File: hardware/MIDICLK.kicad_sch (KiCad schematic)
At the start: 32 parts, among them J1 Conn_02x08_Odd_Even, J2 AudioJack3, J3 AudioJack2, J4 AudioJack2, Q1 2N3904, Q2 2N3904, SW1 RotaryEncoder_Switch, U1 ATtiny85-20P, U2 6N138

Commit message: Assign footprints to components
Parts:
- C1, C2, C3: footprint (none) -> Capacitor_THT:C_Disc_D7.5mm_W5.0mm_P7.50mm
- D2, D3: footprint (none) -> LED_THT:LED_D3.0mm
- J1: footprint (none) -> Connector_IDC:IDC-Header_2x08_P2.54mm_Vertical
- J2: footprint (none) -> AudioJacks:Jack_3.5mm_QingPu_WQP-PJ301CM_Vertical
- J3, J4: footprint (none) -> AudioJacks:Jack_3.5mm_QingPu_WQP-PJ301M-12_Vertical
- R1, R10, R11, R12, R13, R14, R15, R16, R17, R2, R3, R4, R5, R6, R7, R8, R9: footprint (none) -> Resistor_THT:R_Axial_DIN0207_L6.3mm_D2.5mm_P10.16mm_Horizontal
- SW1: footprint (none) -> Rotary_Encoder:RotaryEncoder_Alps_EC11E-Switch_Vertical_H20mm
- U1: footprint Package_DIP:DIP-8_W7.62mm -> Package_DIP:DIP-8_W7.62mm_Socket
- U2: footprint (none) -> Package_DIP:DIP-8_W7.62mm_Socket
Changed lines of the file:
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@@
 			)
 		)
-		(property "Footprint" ""
+		(property "Footprint" "Resistor_THT:R_Axial_DIN0207_L6.3mm_D2.5mm_P10.16mm_Horizontal"
 			(at 210.82 112.268 90)
 			(effects
@@
 			)
 		)
-		(property "Footprint" ""
+		(property "Footprint" "Resistor_THT:R_Axial_DIN0207_L6.3mm_D2.5mm_P10.16mm_Horizontal"
 			(at 210.82 50.038 90)
 			(effects
@@
 			)
 		)
-		(property "Footprint" ""
+		(property "Footprint" "Resistor_THT:R_Axial_DIN0207_L6.3mm_D2.5mm_P10.16mm_Horizontal"
 			(at 244.602 120.65 90)
 			(effects
@@
 			)
 		)
-		(property "Footprint" "Package_DIP:DIP-8_W7.62mm"
+		(property "Footprint" "Package_DIP:DIP-8_W7.62mm_Socket"
 			(at 157.48 82.55 0)
 			(effects
@@
 			)
 		)
-		(property "Footprint" ""
+		(property "Footprint" "Resistor_THT:R_Axial_DIN0207_L6.3mm_D2.5mm_P10.16mm_Horizontal"
 			(at 43.18 91.948 90)
 			(effects
@@
 			)
 		)
-		(property "Footprint" ""
+		(property "Footprint" "Rotary_Encoder:RotaryEncoder_Alps_EC11E-Switch_Vertical_H20mm"
 			(at 82.55 88.646 0)
 			(effects
@@
 			)
 		)
-		(property "Footprint" ""
+		(property "Footprint" "LED_THT:LED_D3.0mm"
 			(at 246.38 48.26 0)
 			(effects
@@
 			)
 		)
-		(property "Footprint" ""
+		(property "Footprint" "Connector_IDC:IDC-Header_2x08_P2.54mm_Vertical"
 			(at 90.17 157.48 0)
 			(effects
@@
 			)
 		)
-		(property "Footprint" ""
+		(property "Footprint" "LED_THT:LED_D3.0mm"
 			(at 246.38 110.49 0)
 			(effects
@@
 			)
 		)
-		(property "Footprint" ""
+		(property "Footprint" "Resistor_THT:R_Axial_DIN0207_L6.3mm_D2.5mm_P10.16mm_Horizontal"
 			(at 89.662 38.1 90)
 			(effects
@@
 			)
 		)
-		(property "Footprint" ""
+		(property "Footprint" "AudioJacks:Jack_3.5mm_QingPu_WQP-PJ301CM_Vertical"
 			(at 34.29 38.1 0)
 			(effects
@@
 			)
 		)
-		(property "Footprint" ""
+		(property "Footprint" "Resistor_THT:R_Axial_DIN0207_L6.3mm_D2.5mm_P10.16mm_Horizontal"
 			(at 100.838 102.87 90)
 			(effects
@@
 			)
 		)
-		(property "Footprint" ""
+		(property "Footprint" "Resistor_THT:R_Axial_DIN0207_L6.3mm_D2.5mm_P10.16mm_Horizontal"
 			(at 48.26 36.322 90)
 			(effects
@@
 			)
 		)
-		(property "Footprint" ""
+		(property "Footprint" "Resistor_THT:R_Axial_DIN0207_L6.3mm_D2.5mm_P10.16mm_Horizontal"
 			(at 67.31 93.472 90)
 			(effects
@@
 			)
 		)
-		(property "Footprint" ""
+		(property "Footprint" "AudioJacks:Jack_3.5mm_QingPu_WQP-PJ301M-12_Vertical"
 			(at 260.35 44.45 0)
 			(effects
@@
 			)
 		)
-		(property "Footprint" ""
+		(property "Footprint" "AudioJacks:Jack_3.5mm_QingPu_WQP-PJ301M-12_Vertical"
 			(at 260.35 106.68 0)
 			(effects
@@
 			)
 		)
-		(property "Footprint" ""
+		(property "Footprint" "Resistor_THT:R_Axial_DIN0207_L6.3mm_D2.5mm_P10.16mm_Horizontal"
 			(at 75.438 83.82 90)
 			(effects
@@
 			)
 		)
-		(property "Footprint" ""
+		(property "Footprint" "Package_DIP:DIP-8_W7.62mm_Socket"
 			(at 82.296 49.53 0)
 			(effects
@@
 			)
 		)
-		(property "Footprint" ""
+		(property "Footprint" "Resistor_THT:R_Axial_DIN0207_L6.3mm_D2.5mm_P10.16mm_Horizontal"
 			(at 235.712 102.87 90)
 			(effects
@@
 			)
 		)
-		(property "Footprint" ""
+		(property "Footprint" "Resistor_THT:R_Axial_DIN0207_L6.3mm_D2.5mm_P10.16mm_Horizontal"
 			(at 223.012 29.21 90)
 			(effects
@@
 			)
 		)
-		(property "Footprint" ""
+		(property "Footprint" "Resistor_THT:R_Axial_DIN0207_L6.3mm_D2.5mm_P10.16mm_Horizontal"
 			(at 223.012 91.44 90)
 			(effects
@@
 			)
 		)
-		(property "Footprint" ""
+		(property "Footprint" "Resistor_THT:R_Axial_DIN0207_L6.3mm_D2.5mm_P10.16mm_Horizontal"
 			(at 47.752 83.82 90)
 			(effects
@@
 			)
 		)
-		(property "Footprint" ""
+		(property "Footprint" "Resistor_THT:R_Axial_DIN0207_L6.3mm_D2.5mm_P10.16mm_Horizontal"
 			(at 244.602 58.42 90)
 			(effects
@@
 			)
 		)
-		(property "Footprint" ""
+		(property "Footprint" "Resistor_THT:R_Axial_DIN0207_L6.3mm_D2.5mm_P10.16mm_Horizontal"
 			(at 235.712 58.42 90)
 			(effects
@@
 			)
 		)
-		(property "Footprint" ""
+		(property "Footprint" "Resistor_THT:R_Axial_DIN0207_L6.3mm_D2.5mm_P10.16mm_Horizontal"
 			(at 235.712 40.64 90)
 			(effects
@@
 			)
 		)
-		(property "Footprint" ""
+		(property "Footprint" "Capacitor_THT:C_Disc_D7.5mm_W5.0mm_P7.50mm"
 			(at 35.8648 106.68 0)
 			(effects
@@
 			)
 		)
-		(property "Footprint" ""
+		(property "Footprint" "Capacitor_THT:C_Disc_D7.5mm_W5.0mm_P7.50mm"
 			(at 139.7 96.8248 0)
 			(effects
@@
 			)
 		)
-		(property "Footprint" ""
+		(property "Footprint" "Capacitor_THT:C_Disc_D7.5mm_W5.0mm_P7.50mm"
 			(at 59.9948 106.68 0)
 			(effects
@@
 			)
 		)
-		(property "Footprint" ""
+		(property "Footprint" "Resistor_THT:R_Axial_DIN0207_L6.3mm_D2.5mm_P10.16mm_Horizontal"
 			(at 235.712 120.65 90)
 			(effects

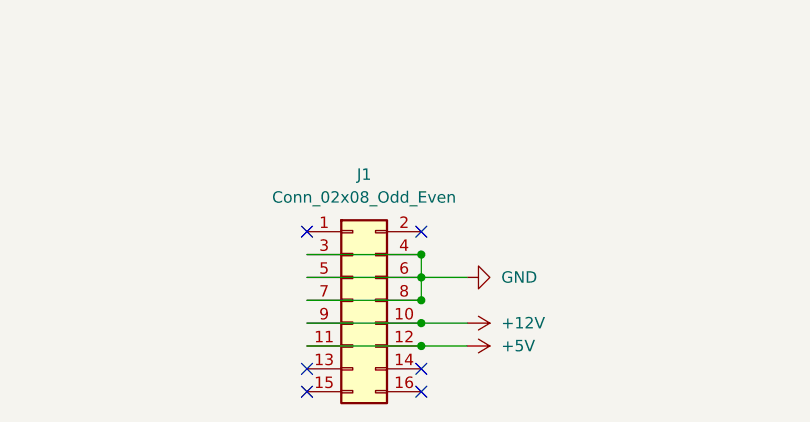
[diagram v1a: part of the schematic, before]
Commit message: Make PCB
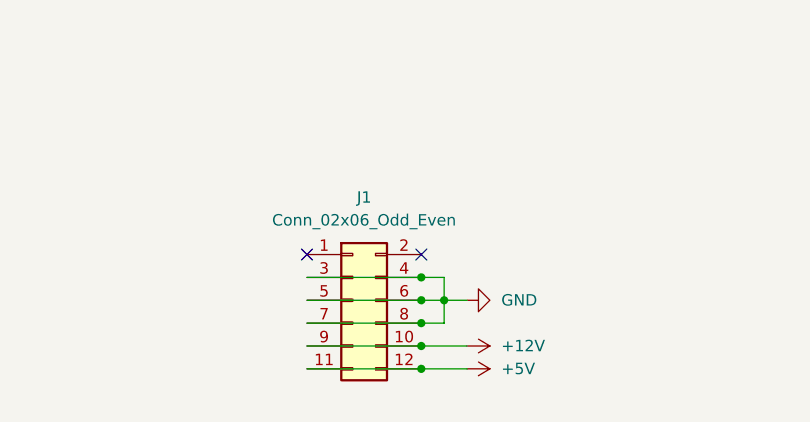
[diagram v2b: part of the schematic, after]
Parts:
- C1, C2, C3: footprint Capacitor_THT:C_Disc_D7.5mm_W5.0mm_P7.50mm -> Capacitor_THT:C_Disc_D5.0mm_W2.5mm_P5.00mm
- J1: value Conn_02x08_Odd_Even -> Conn_02x06_Odd_Even; footprint Connector_IDC:IDC-Header_2x08_P2.54mm_Vertical -> Connector_IDC:IDC-Header_2x06_P2.54mm_Vertical; symbol Connector_Generic:Conn_02x08_Odd_Even -> Connector_Generic:Conn_02x06_Odd_Even
- R1, R10, R11, R12, R13, R14, R15, R16, R17, R2, R3, R4, R5, R6, R7, R8, R9: footprint Resistor_THT:R_Axial_DIN0207_L6.3mm_D2.5mm_P10.16mm_Horizontal -> Resistor_THT:R_Axial_DIN0207_L6.3mm_D2.5mm_P2.54mm_Vertical
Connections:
- no-connect marks 8 -> 4
